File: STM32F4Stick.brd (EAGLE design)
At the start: 46.7 x 25.9 mm, 36 parts, among them U1 MIC5219 3.3V, U2 USD-SOCKETNEW

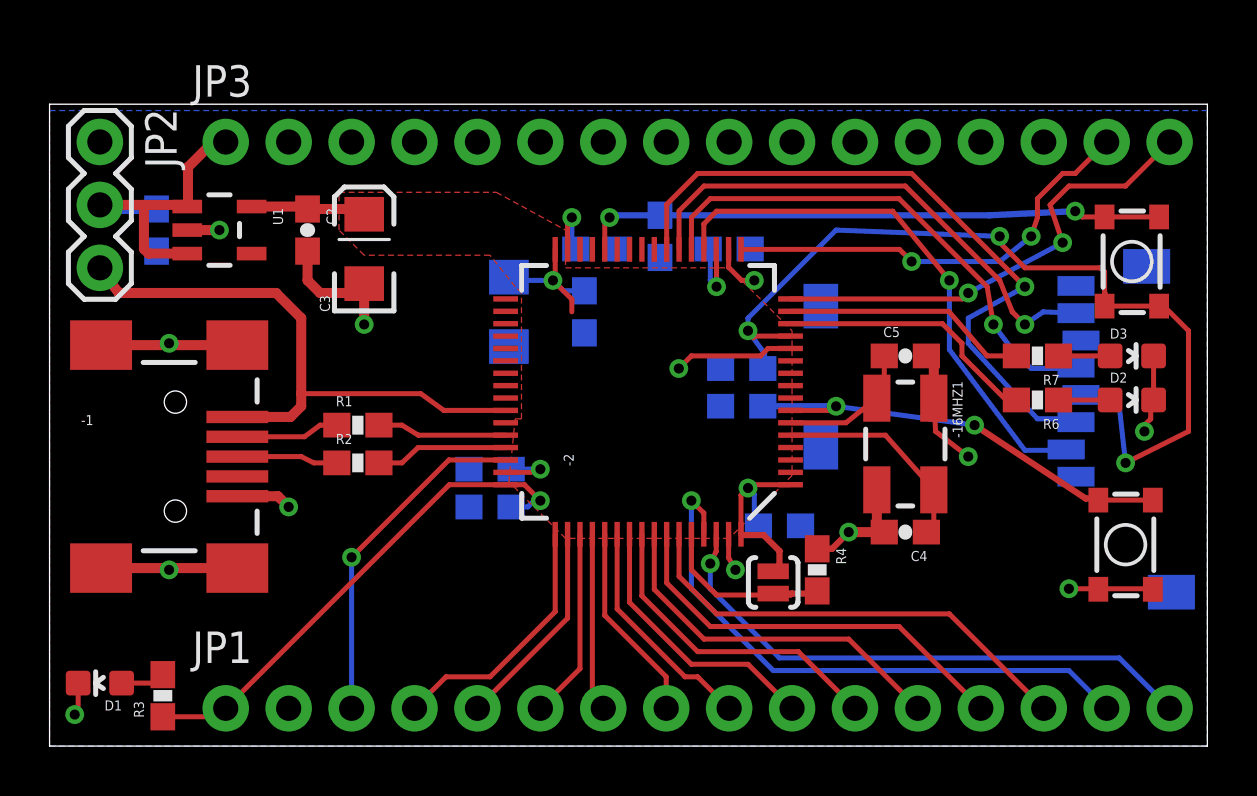
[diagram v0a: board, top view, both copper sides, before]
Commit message: Finished Schematic / Board layout. Silkscreen needs to be added
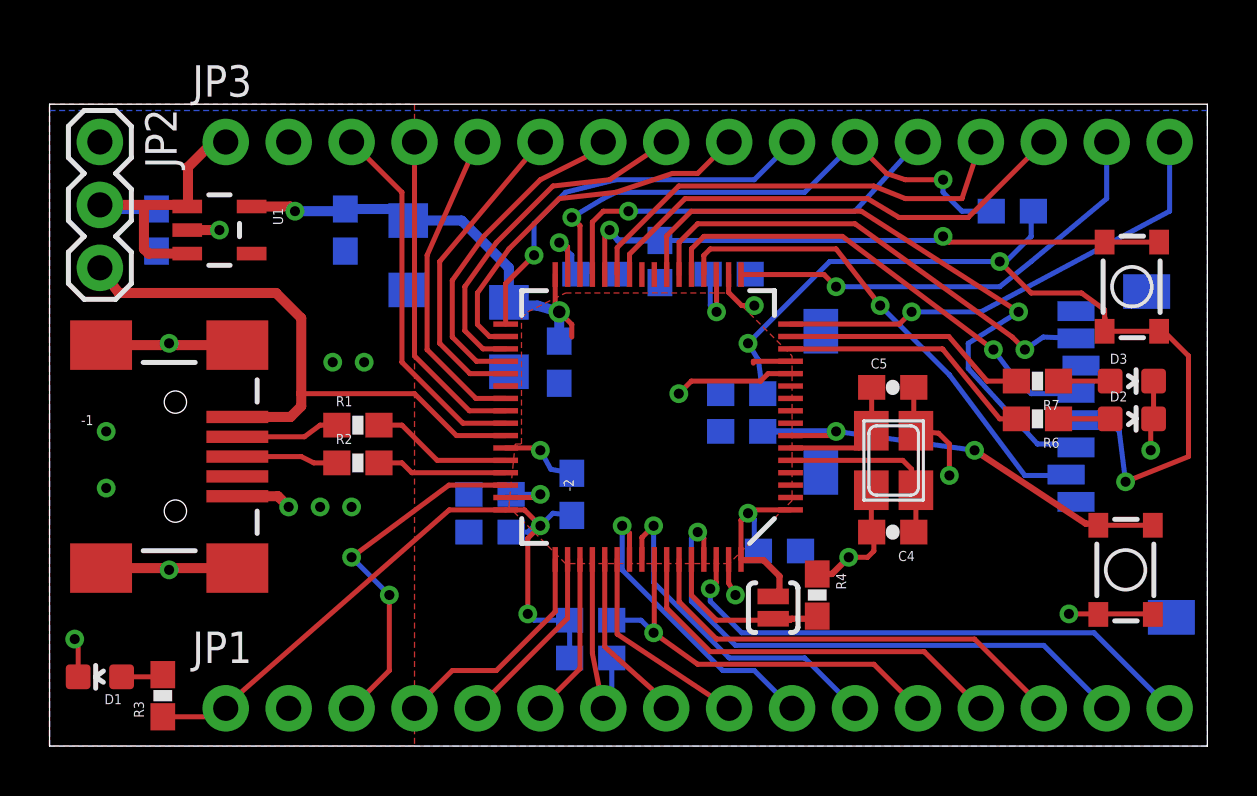
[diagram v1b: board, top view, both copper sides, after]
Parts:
- removed -16MHZ1: CRYSTAL-GROUNDED, SparkFun-FreqCtrl:CRYSTAL-SMD-5X3
- added Q1: (no value), adafruit:NX3225
- added R10, R11, R8, R9: 100k, SparkFun-Resistors:0603-RES
- moved C7 2.27 mm to (20.6, 15.5)
- moved C3 1.80 mm to (14.5, 19.8), flipped to the bottom
- moved C2 1.52 mm to (11.9, 20.8), flipped to the bottom
- moved C5 1.37 mm to (34.0, 14.5)
- moved R5 1.02 mm to (24.6, 19.6)
- moved U2 1.02 mm to (30.7, 18.8)
- moved C11 1.02 mm to (29.5, 7.87)
- moved -2 1.02 mm to (24.2, 13.3)
- moved C10 1.02 mm to (27.9, 14.2)
- moved C13 1.02 mm to (17.8, 10.2)
- moved C14 1.02 mm to (27.9, 12.7)
- moved C9 1.02 mm to (17.8, 8.64)
- moved D3 1.02 mm to (43.7, 14.7)
- moved R4 1.02 mm to (31.0, 6.10)
- moved R7 1.02 mm to (39.9, 14.7)
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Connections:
- removed net N$21: JP3.14
- removed net N$22: JP3.13
- removed net N$23: JP3.12
- removed net N$24: JP3.11
- removed net N$25: JP3.10
- removed net N$26: JP3.9
- removed net N$27: JP3.8
- removed net N$28: JP3.7
- removed net N$29: JP3.6
- removed net N$30: JP3.5
- removed net N$31: JP3.4
- removed net N$32: JP3.3
- new net P26: -2.26, JP3.14
- new net P27: -2.27, JP3.13
- new net P29: -2.29, JP3.12
- new net P30: -2.30, JP3.11, R9.1
- new net P33: -2.33, JP3.10
- new net P34: -2.34, JP3.9
- new net P35: -2.35, JP3.8
- new net P36: -2.36, JP3.7
- new net P37: -2.37, JP3.6
- new net P39: -2.39, JP3.5
- new net P40: -2.40, JP3.4
- new net P41: -2.41, JP3.3
- net GND: now also Q1.2, Q1.4; no longer -16MHZ1.2, -16MHZ1.4
- net N$3: now also Q1.1; no longer -16MHZ1.3
- net N$4: now also Q1.3; no longer -16MHZ1.1
- net P52: now also R10.1
- net P57: now also R11.1
- net USB_ID: now also R8.1
- net VCC: now also R10.2, R11.2, R8.2, R9.2
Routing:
- net P30: track 0.00 -> 21.9 mm, vias 0 -> 2
- net P26: track 0.00 -> 19.9 mm
- net P27: track 0.00 -> 18.5 mm
- net VCC: track 80.9 -> 98.9 mm, vias 7 -> 9
- net P29: track 0.00 -> 16.7 mm, vias 0 -> 1
- net P33: track 0.00 -> 16.2 mm, vias 0 -> 1
- net P34: track 0.00 -> 15.2 mm
- net P41: track 0.00 -> 14.9 mm
- net P35: track 0.00 -> 14.2 mm
- net P36: track 0.00 -> 13.4 mm
- net P40: track 0.00 -> 13.2 mm
- net P39: track 0.00 -> 12.8 mm
- net P37: track 0.00 -> 12.8 mm
- net GND: track 47.0 -> 41.4 mm, vias 13 -> 18
- net USB_ID: track 0.00 -> 3.18 mm, vias 0 -> 1
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- added copper zone on layer 1, net GND
